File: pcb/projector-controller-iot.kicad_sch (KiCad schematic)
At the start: 33 parts, among them J1 DE9_Pins, J2 USB_C_Receptacle, J3 Conn_01x04_Socket, J4 Conn_01x04_Socket, J5 Barrel_Jack, SW1 SW_Push, U1 ESP32-S3-WROOM-1, U2 SP3232EEN-L/TR, U3 LP5907MFX-3.3

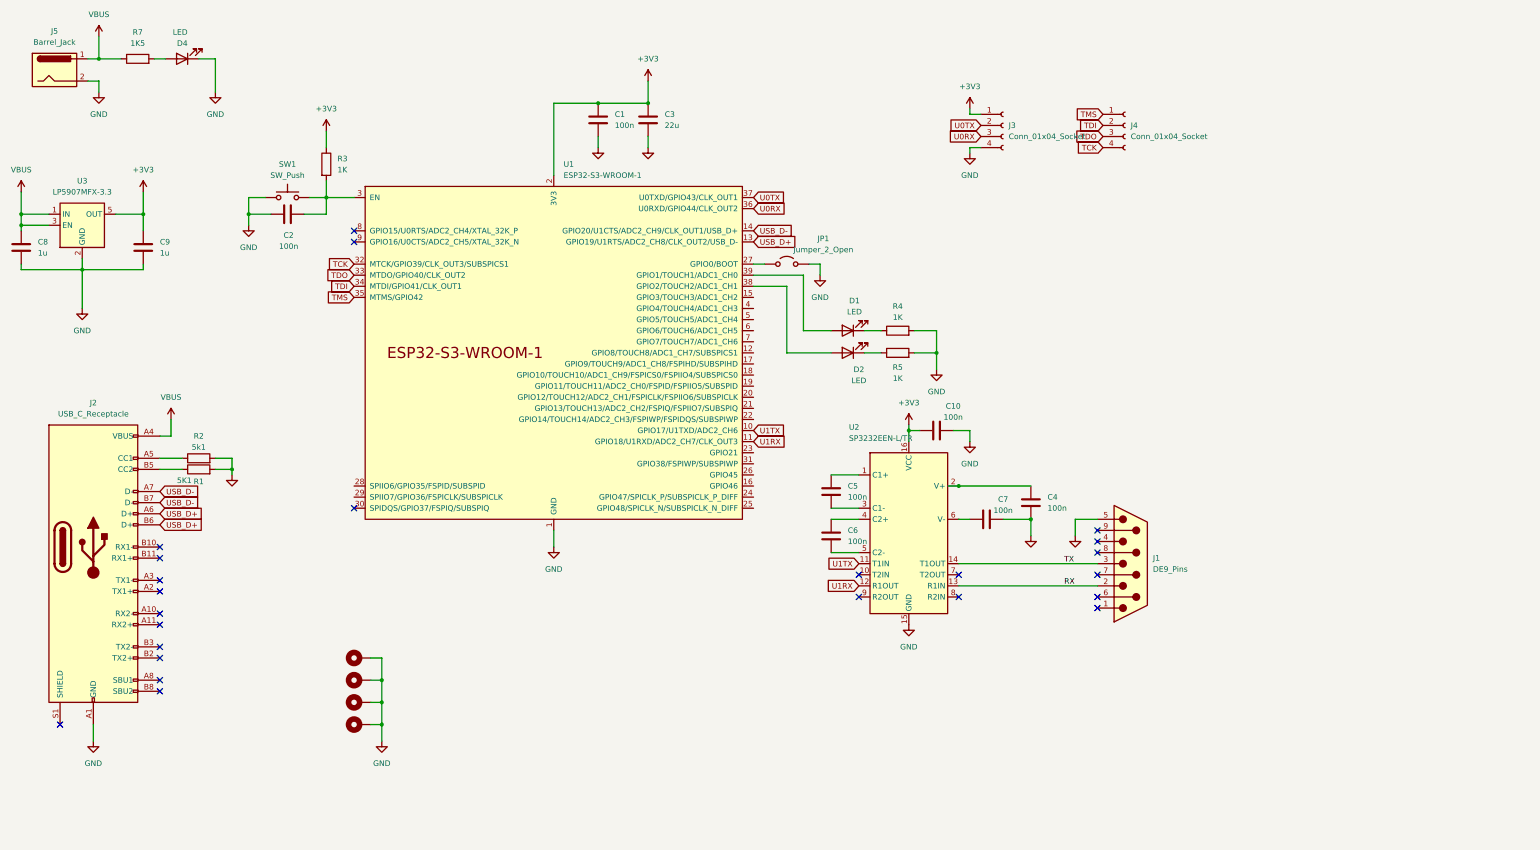
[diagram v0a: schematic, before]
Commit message: Bro idk
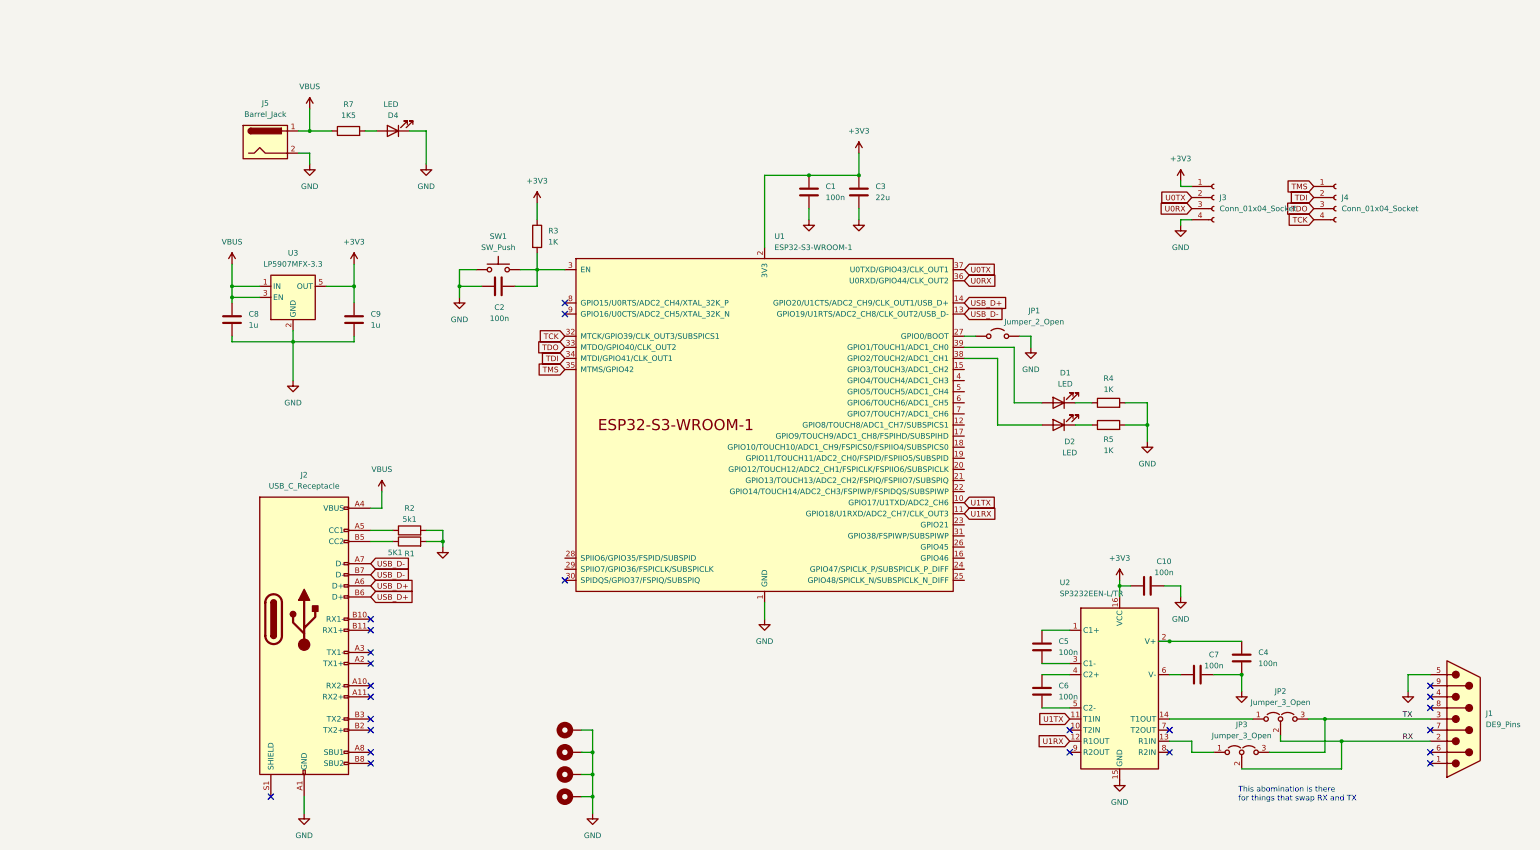
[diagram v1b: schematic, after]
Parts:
- added JP2, JP3: Jumper_3_Open, symbol Jumper:Jumper_3_Open
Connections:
- net RX: now also JP2.2 (C), JP3.2 (C); no longer U2.13 (R1IN)
- net TX: now also JP2.3 (B), JP3.3 (B); no longer U2.14 (T1OUT)
- net USB_D+: now also U1.14 (GPIO20/U1CTS/ADC2_CH9/CLK_OUT1/USB_D+); no longer U1.13 (GPIO19/U1RTS/ADC2_CH8/CLK_OUT2/USB_D-)
- net USB_D-: now also U1.13 (GPIO19/U1RTS/ADC2_CH8/CLK_OUT2/USB_D-); no longer U1.14 (GPIO20/U1CTS/ADC2_CH9/CLK_OUT1/USB_D+)
- new net: JP3.1 (A), U2.13 (R1IN)
- new net: JP2.1 (A), U2.14 (T1OUT)
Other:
- note added: "This abomination is there for things that swap RX and TX"
- moved on the sheet: C1, C10, C2, C3, C4, C5, C6, C7, C8, C9, D1, D2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
